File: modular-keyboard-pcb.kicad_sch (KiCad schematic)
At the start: 8 parts, among them J1 Conn_01x02, J2 mag_pogo_01x05, J3 mag_pogo_01x05, J4 mag_pogo_01x05, J5 mag_pogo_01x05, SW1 SW_Push, SW2 SW_Wuerth_450301014042, U1 nice_nano

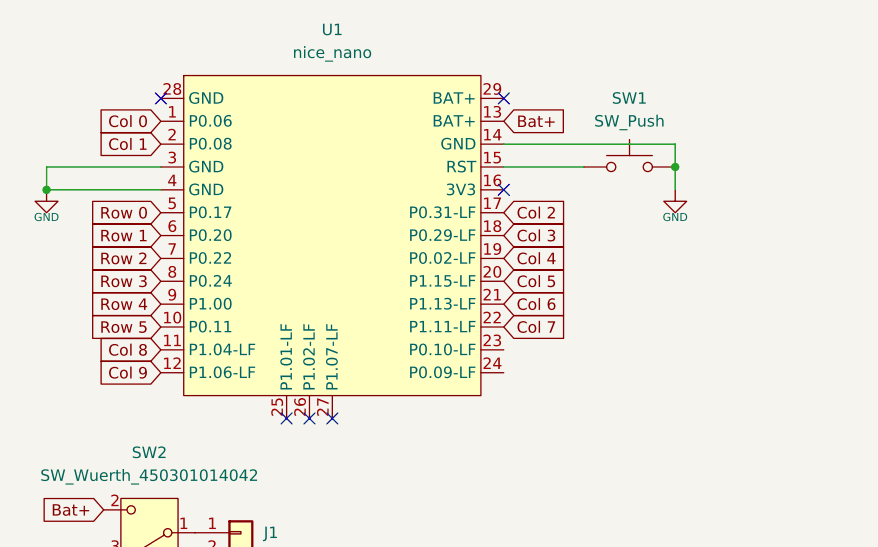
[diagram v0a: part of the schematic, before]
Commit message: day 3
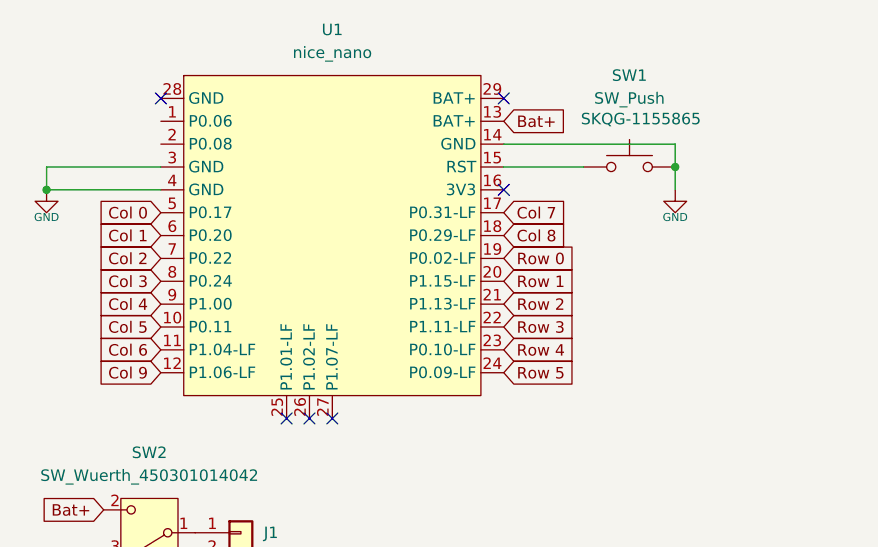
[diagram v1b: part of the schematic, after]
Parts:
- SW1: footprint (none) -> SKQG-1155865
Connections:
- net Col 0: now also U1.5 (P0.17); no longer U1.1 (P0.06)
- net Col 1: now also U1.6 (P0.20); no longer U1.2 (P0.08)
- net Col 2: now also U1.7 (P0.22); no longer U1.17 (P0.31-LF)
- net Col 3: now also U1.8 (P0.24); no longer U1.18 (P0.29-LF)
- net Col 4: now also U1.9 (P1.00); no longer U1.19 (P0.02-LF)
- net Col 5: now also U1.10 (P0.11); no longer U1.20 (P1.15-LF)
- net Col 6: now also U1.11 (P1.04-LF); no longer U1.21 (P1.13-LF)
- net Col 7: now also U1.17 (P0.31-LF); no longer U1.22 (P1.11-LF)
- net Col 8: now also U1.18 (P0.29-LF); no longer U1.11 (P1.04-LF)
- net Row 0: now also U1.19 (P0.02-LF); no longer U1.5 (P0.17)
- net Row 1: now also U1.20 (P1.15-LF); no longer U1.6 (P0.20)
- net Row 2: now also U1.21 (P1.13-LF); no longer U1.7 (P0.22)
- net Row 3: now also U1.22 (P1.11-LF); no longer U1.8 (P0.24)
- net Row 4: now also U1.23 (P0.10-LF); no longer U1.9 (P1.00)
- net Row 5: now also U1.24 (P0.09-LF); no longer U1.10 (P0.11)
